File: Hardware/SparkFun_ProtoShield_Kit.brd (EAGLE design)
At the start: 53.3 x 67.3 mm, 29 parts

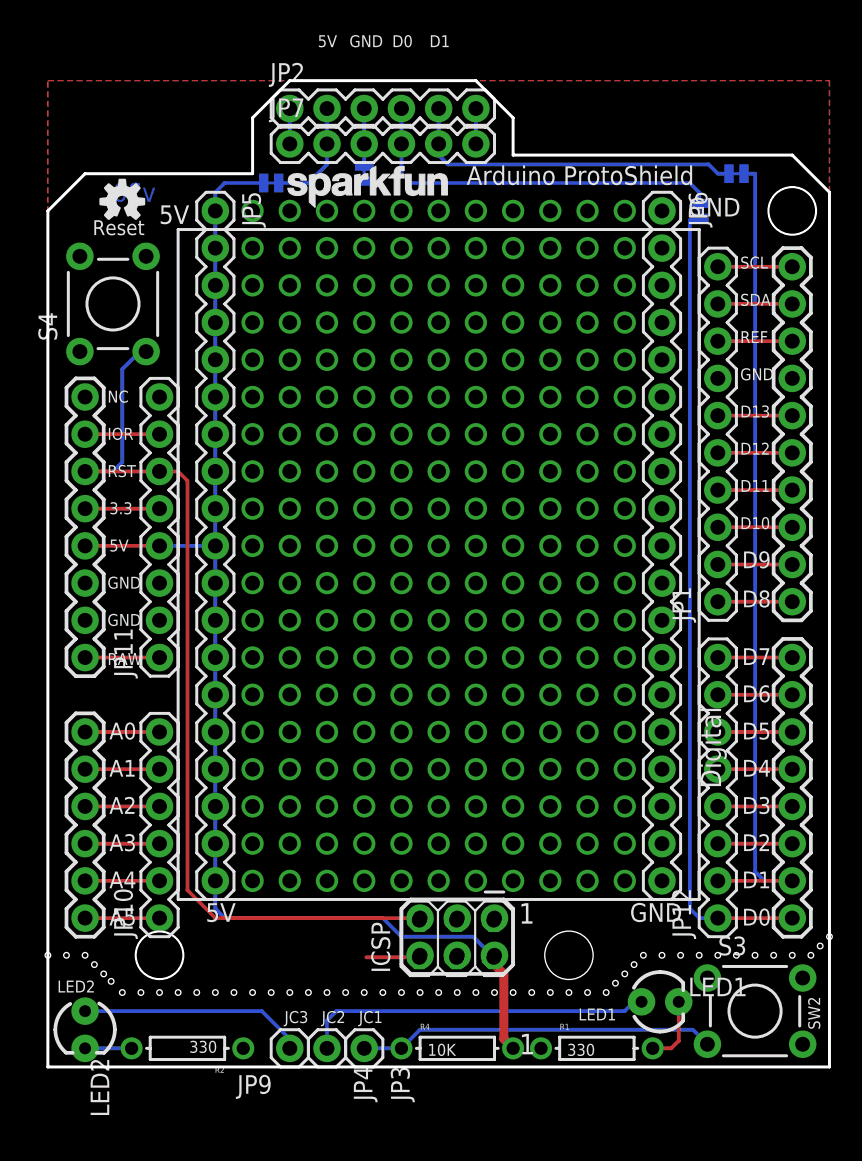
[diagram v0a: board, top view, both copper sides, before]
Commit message: Updates from engineering review
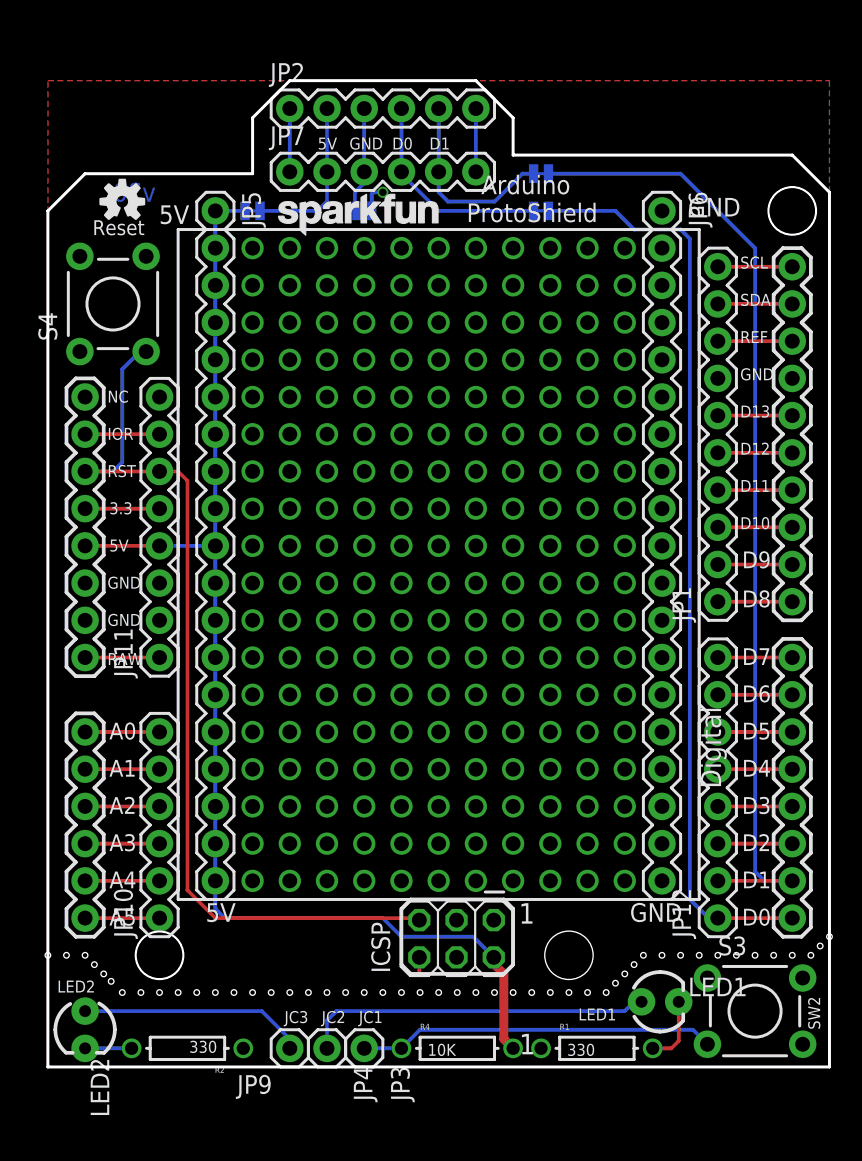
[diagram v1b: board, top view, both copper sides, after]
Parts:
- moved SJ1 13.3 mm to (33.7, 61.0)
- moved SJ2 10.8 mm to (33.7, 58.4), turned to 180 degrees
- moved SJ3 2.54 mm to (21.6, 58.4), turned to 180 degrees
- moved SJ4 2.29 mm to (14.0, 58.4)
- moved U$1 2.01 mm to (15.2, 56.3)
- moved JP7 1.90 mm to (16.5, 61.1)
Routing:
- net FTDI_RX: track 26.1 -> 14.5 mm
- net TX: track 56.3 -> 66.6 mm
- net FTDI_TX: track 23.5 -> 13.2 mm
- net RX: track 55.0 -> 63.7 mm
- net FTDI_5V: track 7.64 -> 11.2 mm
- net FTDI_GND: track 3.94 -> 7.30 mm
- net 5V: track 88.5 -> 85.7 mm
- net NC2: track 2.41 -> 4.32 mm
- net NC1: track 2.41 -> 4.32 mm
- net GND: track 3.62 -> 3.11 mm, vias 0 -> 1
- removed copper zone on layer 16, net GND

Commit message: WIP-bumping annular rings
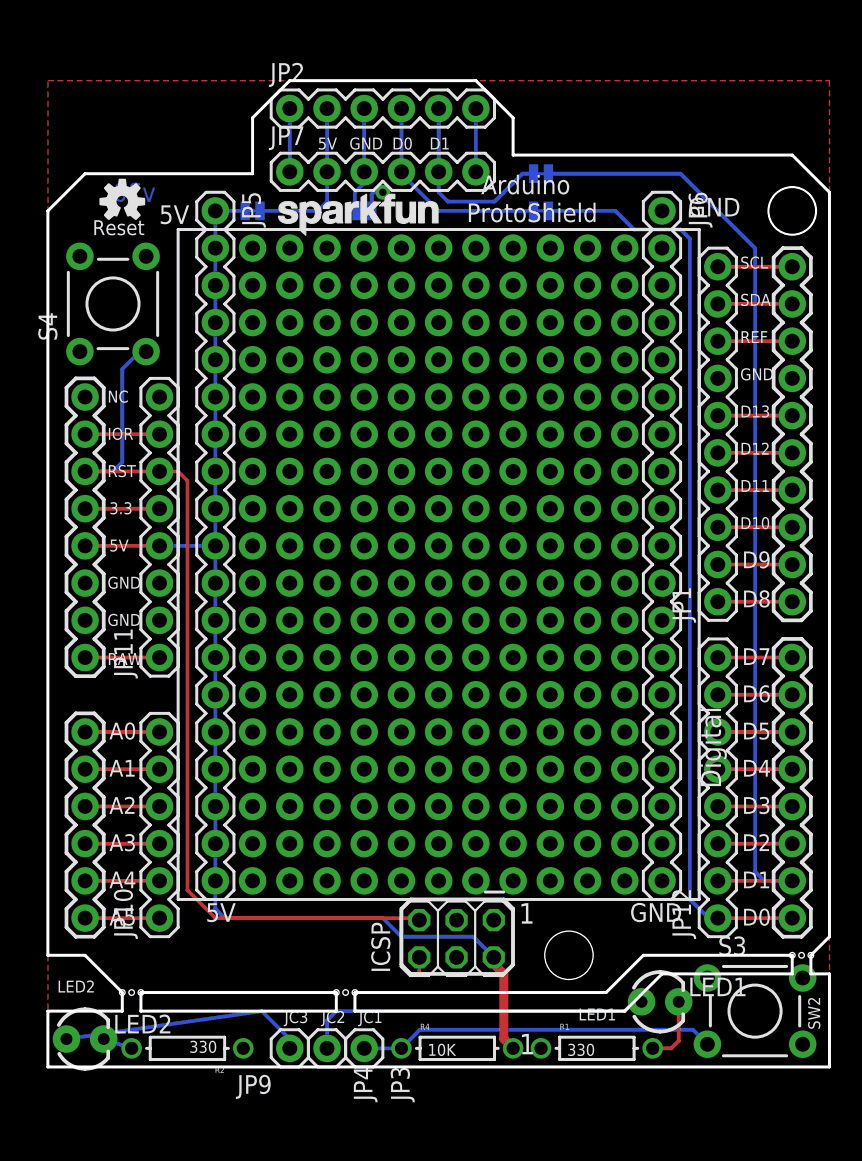
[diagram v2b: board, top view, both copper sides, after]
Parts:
- moved LED2 0.64 mm to (2.54, 1.91), turned to 0 degrees
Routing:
- net LED2: track 15.4 -> 16.8 mm
- net N$7: track 3.17 -> 2.01 mm
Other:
- outline, holes or cut-outs redrawn

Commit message: Updates from checklist
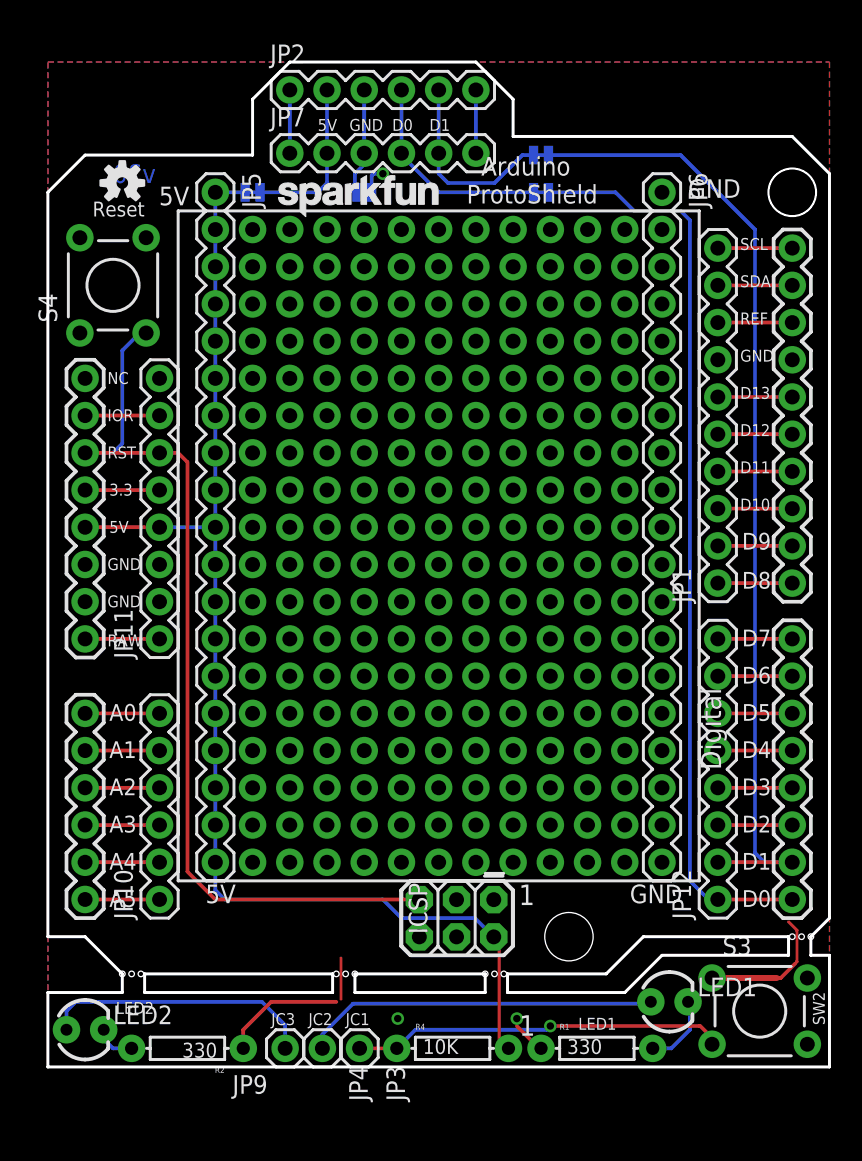
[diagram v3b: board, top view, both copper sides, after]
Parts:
- BB1: device SparkFun:BREADBOARD-MINI -> SparkFun-Boards:BREADBOARD-MINI
- ICSP: device pinhead:2X03 -> SparkFun-Connectors:2X3
- R1, R2, R4: device SparkFun:AXIAL-0.3 -> SparkFun-Resistors:AXIAL-0.3
- moved ICSP 3.68 mm to (30.4, 11.4)
- moved JP8 1.27 mm to (53.3, 66.0)
- moved BB1 1.27 mm to (8.89, 58.4)
- moved JP1 1.27 mm to (45.7, 33.0)
- moved LOGO1 1.27 mm to (5.08, 60.3)
- moved S4 1.27 mm to (4.45, 53.3)
- moved FRAME1 1.27 mm to (1.80, -14.6)
- moved JP10 1.27 mm to (7.62, 11.4)
- moved JP11 1.27 mm to (7.62, 29.2)
- moved JP12 1.27 mm to (45.7, 11.4)
- moved U$2 1.27 mm to (13.3, -17.1)
- moved JP2 1.27 mm to (16.5, 66.7)
- moved JP5 1.27 mm to (11.4, 59.7)
- moved JP6 1.27 mm to (41.9, 59.7)
- moved JP7 1.27 mm to (16.5, 62.4)
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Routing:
- net GND: track 3.11 -> 24.7 mm, vias 1 -> 3
- net LED2: track 16.8 -> 18.7 mm
- net 5V: track 85.7 -> 86.9 mm
- net RES: track 24.4 -> 25.5 mm, vias 0 -> 1
- net N$7: track 2.01 -> 2.80 mm
- added copper zone on layer 16, net GND
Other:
- board size 53.3 x 67.3 mm -> 53.3 x 68.6 mm
- board text added: "RX"
- board text added: "TX"
